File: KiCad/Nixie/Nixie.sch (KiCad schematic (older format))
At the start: 31 parts, among them J1 Screw_Terminal_01x02, J2 DB9_Male_MountingHoles, J3 DB9_Female_MountingHoles, Q1 MMBTA42, Q10 MMBTA42, Q2 MMBTA42, Q3 MMBTA42, Q4 MMBTA42, Q5 MMBTA42, Q6 MMBTA42, Q7 MMBTA42, Q8 MMBTA42, Q9 MMBTA42, U1 74HC595, U2 4028

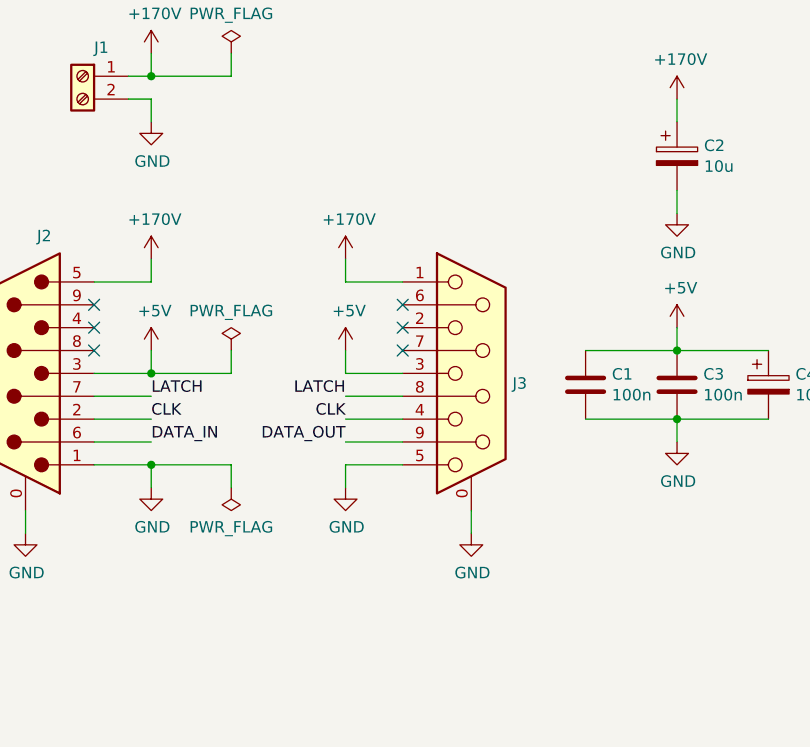
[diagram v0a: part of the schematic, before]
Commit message: PCB routing part 1
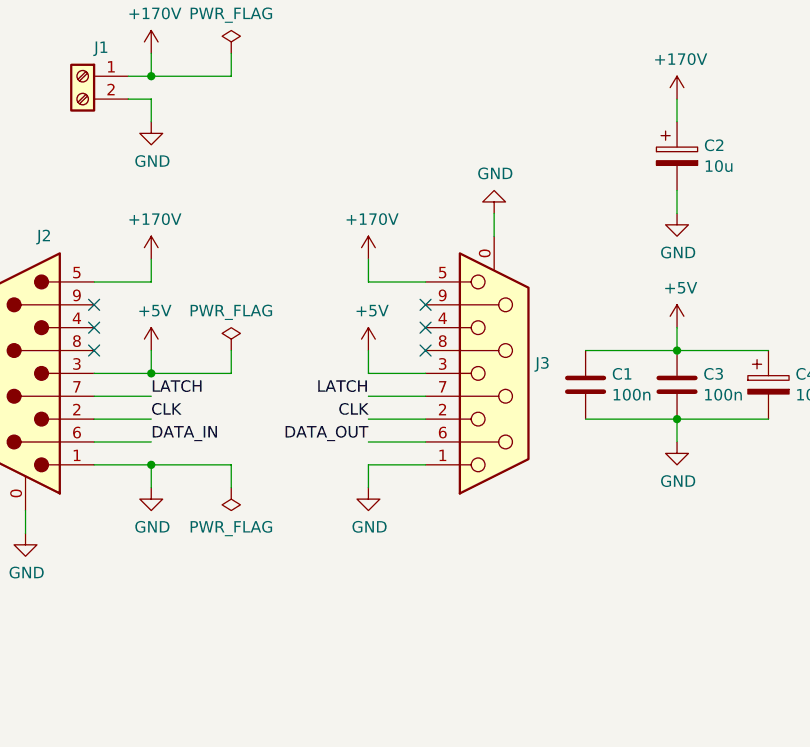
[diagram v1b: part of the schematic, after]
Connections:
- net +170V: now also J3.5; no longer J3.1
- net CLK: now also J3.2; no longer J3.4
- net DATA_OUT: now also J3.6; no longer J3.9
- net GND: now also J3.1; no longer J3.5
- net LATCH: now also J3.7; no longer J3.8
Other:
- moved on the sheet: J3
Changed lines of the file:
@@
 L power:+5V #PWR?
 U 1 1 5D560501
-P 2500 2300
-F 0 "#PWR?" H 2500 2150 50  0001 C CNN
-F 1 "+5V" H 2515 2473 50  0000 C CNN
-F 2 "" H 2500 2300 50  0001 C CNN
-F 3 "" H 2500 2300 50  0001 C CNN
-	1    2500 2300
+P 2600 2300
+F 0 "#PWR?" H 2600 2150 50  0001 C CNN
+F 1 "+5V" H 2615 2473 50  0000 C CNN
+F 2 "" H 2600 2300 50  0001 C CNN
+F 3 "" H 2600 2300 50  0001 C CNN
+	1    2600 2300
 	1    0    0    -1
 $EndComp
@@
 L power:GND #PWR?
 U 1 1 5D560BCA
-P 2500 2900
-F 0 "#PWR?" H 2500 2650 50  0001 C CNN
-F 1 "GND" H 2505 2727 50  0000 C CNN
-F 2 "" H 2500 2900 50  0001 C CNN
-F 3 "" H 2500 2900 50  0001 C CNN
-	1    2500 2900
-	1    0    0    -1
-$EndComp
-Wire Wire Line
-	2500 2800 2500 2900
-Wire Wire Line
-	2500 2400 2500 2300
+P 2600 2900
+F 0 "#PWR?" H 2600 2650 50  0001 C CNN
+F 1 "GND" H 2605 2727 50  0000 C CNN
+F 2 "" H 2600 2900 50  0001 C CNN
+F 3 "" H 2600 2900 50  0001 C CNN
+	1    2600 2900
+	1    0    0    -1
+$EndComp
+Wire Wire Line
+	2600 2000 2600 1900
 Wire Wire Line
 	2950 5200 3350 5200
@@
 Text Label 1650 2700 0    50   ~ 0
 DATA_IN
-Text Label 2500 2700 2    50   ~ 0
+Text Label 2600 2700 2    50   ~ 0
 DATA_OUT
-Text Label 2500 2600 2    50   ~ 0
+Text Label 2600 2600 2    50   ~ 0
 CLK
-Text Label 2500 2500 2    50   ~ 0
+Text Label 2600 2500 2    50   ~ 0
 LATCH
 $Comp
@@
 L Nixie-rescue:+170V-power #PWR?
 U 1 1 5D60968C
-P 2500 1900
-F 0 "#PWR?" H 2500 1750 50  0001 C CNN
-F 1 "+170V" H 2515 2073 50  0000 C CNN
-F 2 "" H 2500 1900 50  0001 C CNN
-F 3 "" H 2500 1900 50  0001 C CNN
-	1    2500 1900
-	1    0    0    -1
-$EndComp
-Wire Wire Line
-	2500 1900 2500 2000
+P 2600 1900
+F 0 "#PWR?" H 2600 1750 50  0001 C CNN
+F 1 "+170V" H 2615 2073 50  0000 C CNN
+F 2 "" H 2600 1900 50  0001 C CNN
+F 3 "" H 2600 1900 50  0001 C CNN
+	1    2600 1900
+	1    0    0    -1
+$EndComp
+Wire Wire Line
+	2600 2900 2600 2800
 $Comp
 L Nixie-rescue:+170V-power #PWR?
@@
 Connection ~ 1650 2800
 $Comp
-L Connector:DB9_Female_MountingHoles J3
-U 1 1 5D3FDF15
-P 3050 2400
-F 0 "J3" H 3230 2356 50  0000 L CNN
-F 1 "DB9_Female_MountingHoles" H 3230 2311 50  0001 L CNN
-F 2 "Connector_Dsub:DSUB-9_Male_Horizontal_P2.77x2.84mm_EdgePinOffset7.70mm_Housed_MountingHolesOffset9.12mm" H 3050 2400 50  0001 C CNN
-F 3 " ~" H 3050 2400 50  0001 C CNN
-	1    3050 2400
-	1    0    0    -1
-$EndComp
-$Comp
 L Connector:DB9_Male_MountingHoles J2
 U 1 1 5D406C9F
@@
 L power:GND #PWR?
 U 1 1 5D4476A3
-P 3050 3100
-F 0 "#PWR?" H 3050 2850 50  0001 C CNN
-F 1 "GND" H 3055 2927 50  0000 C CNN
-F 2 "" H 3050 3100 50  0001 C CNN
-F 3 "" H 3050 3100 50  0001 C CNN
-	1    3050 3100
-	1    0    0    -1
-$EndComp
-Wire Wire Line
-	3050 3100 3050 3000
+P 3150 1700
+F 0 "#PWR?" H 3150 1450 50  0001 C CNN
+F 1 "GND" H 3155 1527 50  0000 C CNN
+F 2 "" H 3150 1700 50  0001 C CNN
+F 3 "" H 3150 1700 50  0001 C CNN
+	1    3150 1700
+	1    0    0    1
+$EndComp
+Wire Wire Line
+	3150 1700 3150 1800
 Wire Wire Line
 	1400 2800 1650 2800
 Wire Wire Line
-	2500 2800 2750 2800
-Wire Wire Line
-	2500 2700 2750 2700
-Wire Wire Line
-	2500 2600 2750 2600
-Wire Wire Line
-	2500 2500 2750 2500
-Wire Wire Line
-	2500 2400 2750 2400
+	2600 2000 2850 2000
 Wire Wire Line
 	1400 2700 1650 2700
@@
 	1400 2000 1650 2000
 Wire Wire Line
-	2500 2000 2750 2000
+	2600 2800 2850 2800
 NoConn ~ 1400 2100
 NoConn ~ 1400 2200
 NoConn ~ 1400 2300
-NoConn ~ 2750 2100
-NoConn ~ 2750 2200
-NoConn ~ 2750 2300
+$Comp
+L Connector:DB9_Female_MountingHoles J3
+U 1 1 5D3FDF15
+P 3150 2400
+F 0 "J3" H 3330 2356 50  0000 L CNN
+F 1 "DB9_Female_MountingHoles" H 3330 2311 50  0001 L CNN
+F 2 "Connector_Dsub:DSUB-9_Male_Horizontal_P2.77x2.84mm_EdgePinOffset7.70mm_Housed_MountingHolesOffset9.12mm" H 3150 2400 50  0001 C CNN
+F 3 " ~" H 3150 2400 50  0001 C CNN
+	1    3150 2400
+	1    0    0    1
+$EndComp
+Wire Wire Line
+	2600 2300 2600 2400
+Wire Wire Line
+	2600 2400 2850 2400
+Wire Wire Line
+	2850 2500 2600 2500
+Wire Wire Line
+	2600 2600 2850 2600
+Wire Wire Line
+	2850 2700 2600 2700
+NoConn ~ 2850 2100
+NoConn ~ 2850 2200
+NoConn ~ 2850 2300
 $EndSCHEMATC
